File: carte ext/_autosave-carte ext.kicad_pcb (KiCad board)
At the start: 2 copper layers, 86.7 x 56.6 mm, 341 parts, among them J1 Conn_01x02, J10 Conn_01x04, J11 Conn_01x04, J12 Conn_01x04, J13 Conn_01x04, J14 Conn_01x04, J15 Conn_01x04, J16 Conn_01x04, J17 Conn_01x04, J18 Conn_01x04, J19 Conn_01x04, J2 Conn_01x02, J20 Conn_01x04, J21 Conn_02x04_Odd_Even, J22 Conn_02x04_Odd_Even, J23 Conn_02x04_Odd_Even, J24 Conn_02x04_Odd_Even, J25 Conn_02x04_Odd_Even, J26 Conn_02x04_Odd_Even, J27 Conn_02x04_Odd_Even, J28 Conn_02x04_Odd_Even, J29 Conn_02x04_Odd_Even, J3 Conn_01x04, J30 Conn_02x04_Odd_Even, J31 Conn_02x04_Odd_Even, J32 Conn_02x04_Odd_Even, J33 Conn_01x02, J4 Conn_01x04, J5 Conn_01x04, J6 Conn_01x04, J7 Conn_01x04, J8 Conn_01x04, J9 Conn_01x04, U1 PCA9685PW, U2 PCA9685PW, U3 PCA9685PW, U4 PCF8574AT, U5 PCF8574AT

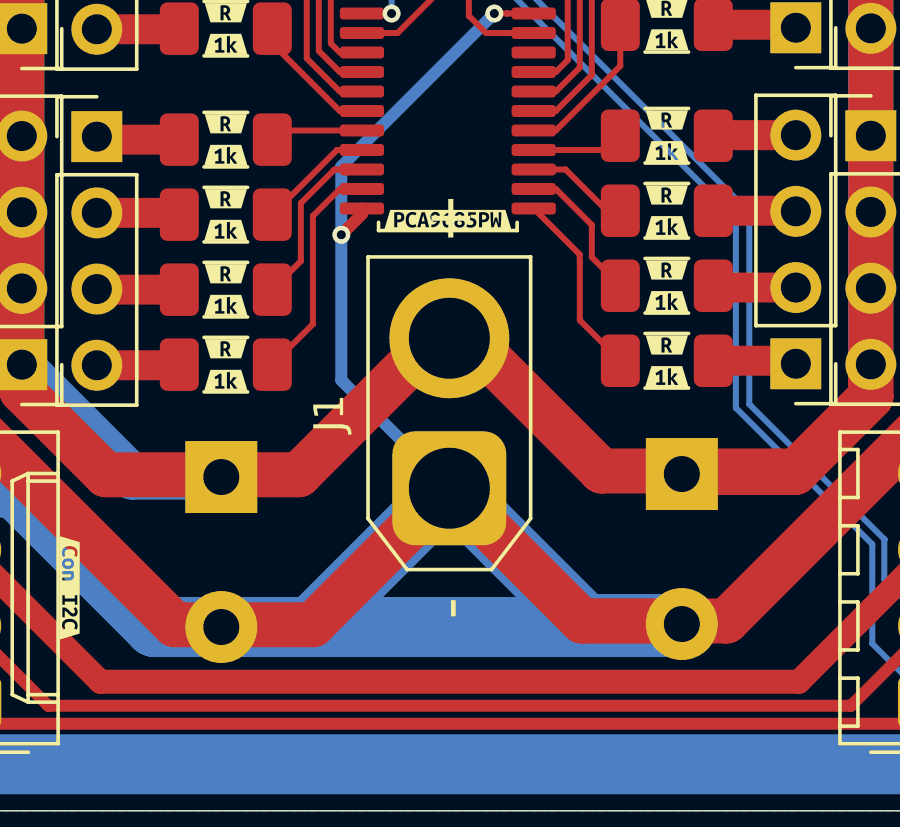
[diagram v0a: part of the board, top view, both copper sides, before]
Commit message: xt30
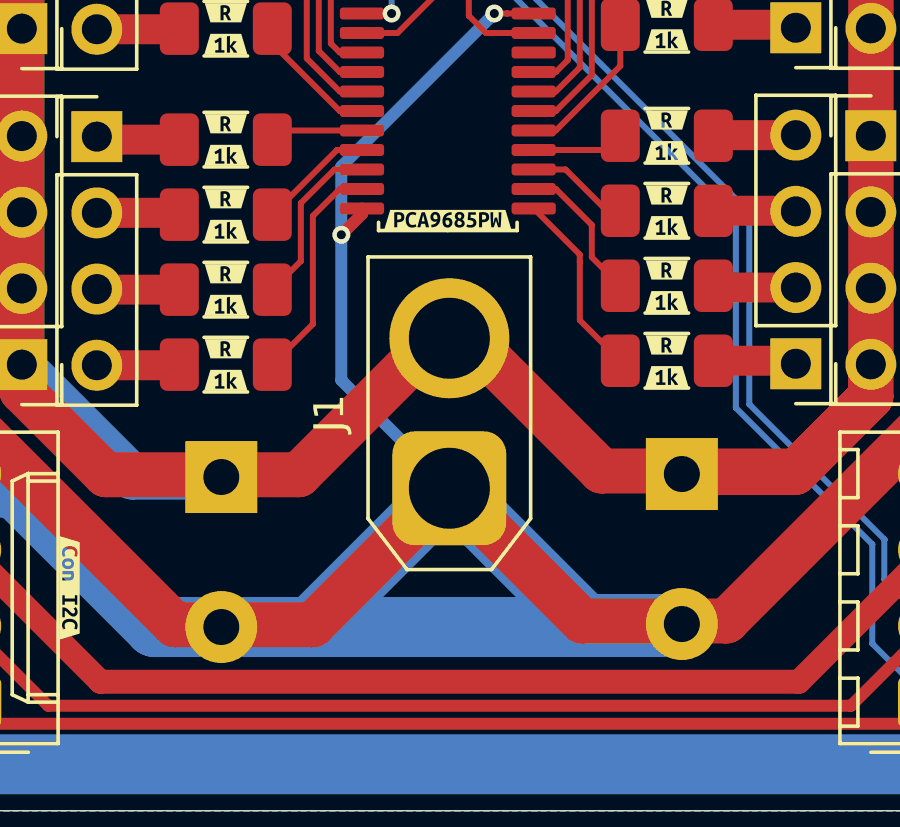
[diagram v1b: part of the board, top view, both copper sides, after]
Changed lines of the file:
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@@
 			(layer "F.Fab")
-		)
-		(fp_text user "+"
-			(at 9 0 90)
-			(layer "F.SilkS")
-			(effects
-				(font
-					(size 1.5 1.5)
-					(thickness 0.15)
-				)
-			)
-		)
-		(fp_text user "-"
-			(at -4 0 90)
-			(layer "F.SilkS")
-			(effects
-				(font
-					(size 1.5 1.5)
-					(thickness 0.15)
-				)
-			)
 		)
 		(fp_text user "${REFERENCE}"
